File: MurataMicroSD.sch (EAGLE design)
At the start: 9 parts, among them U1 IC_BLE_LBCA2HNZYZ-711

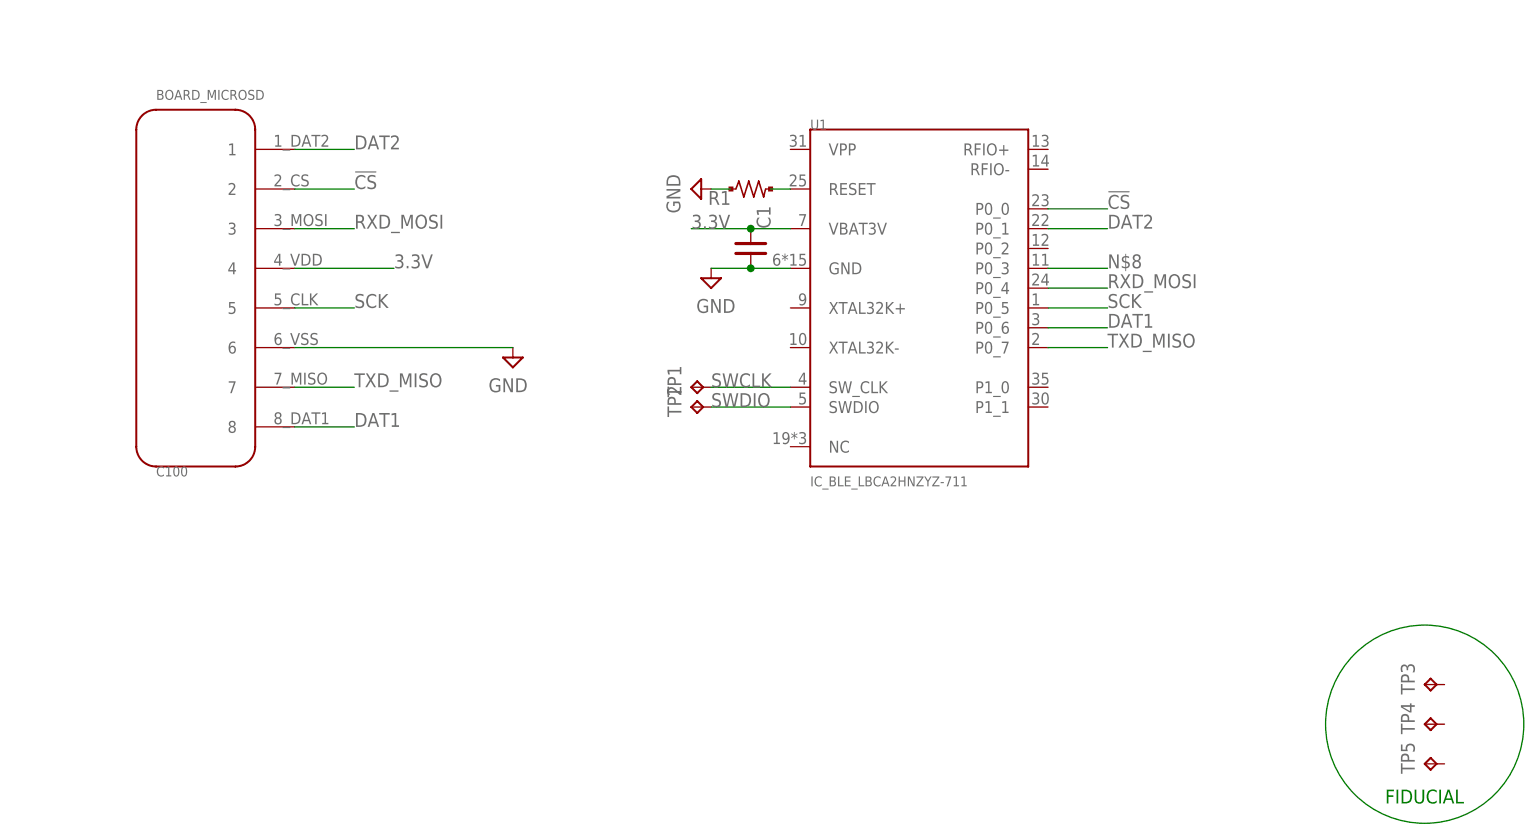
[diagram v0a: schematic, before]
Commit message: [ FIX ] SCH change; library update myPCBlib: 385519d7d8f28a1be9991780ecc3cf499a6be8e2
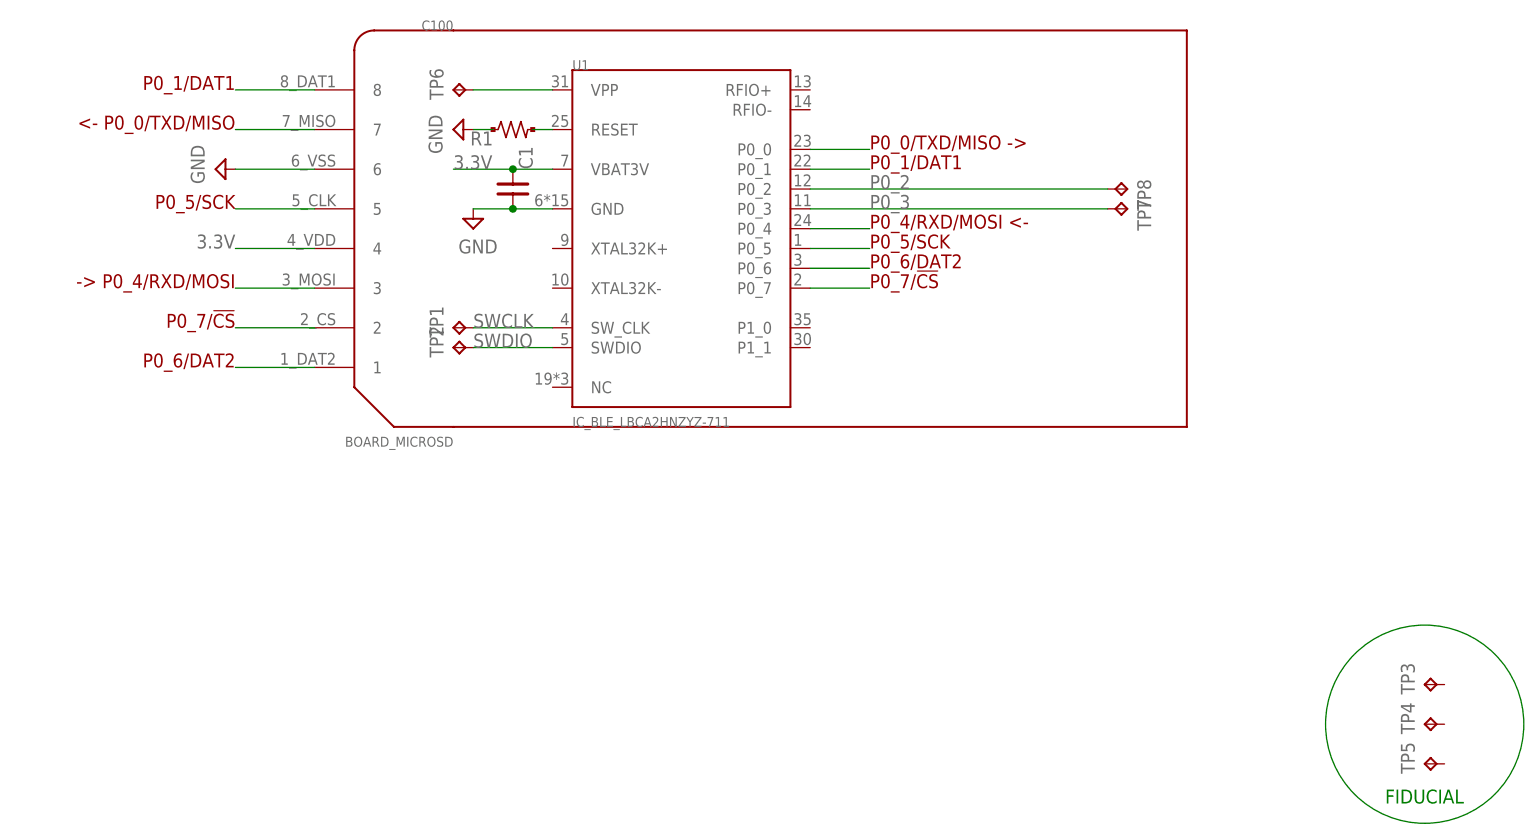
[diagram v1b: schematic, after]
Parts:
- added TP6, TP7, TP8: TPTP08R, testpad_local:TPTP08R
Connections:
- removed net N$8: U1.P0_3
- removed net TXD_MISO: C100.7, U1.P0_7
- new net MISO: C100.7, U1.P0_0
- new net N$2: TP6.TP, U1.VPP
- new net P0_2: TP8.TP, U1.P0_2
- new net P0_3: TP7.TP, U1.P0_3
- net !CS!: now also U1.P0_7; no longer U1.P0_0
- net DAT1: now also U1.P0_1; no longer U1.P0_6
- net DAT2: now also U1.P0_6; no longer U1.P0_1
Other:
- note added: "-> P0_4/RXD/MOSI"
- note added: "<- P0_0/TXD/MISO"
- note added: "P0_0/TXD/MISO ->"
- note added: "P0_1/DAT1"
- note added: "P0_4/RXD/MOSI <-"
- note added: "P0_5/SCK"
- note added: "P0_6/DAT2"
- note added: "P0_7/!CS!"
- moved on the sheet: C1, R1, TP1, TP2, U1
